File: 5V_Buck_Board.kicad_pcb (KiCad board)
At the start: 2 copper layers, 97.1 x 70 mm, 10 parts, among them J1 XT60PW-M, J2 XT60PW-F

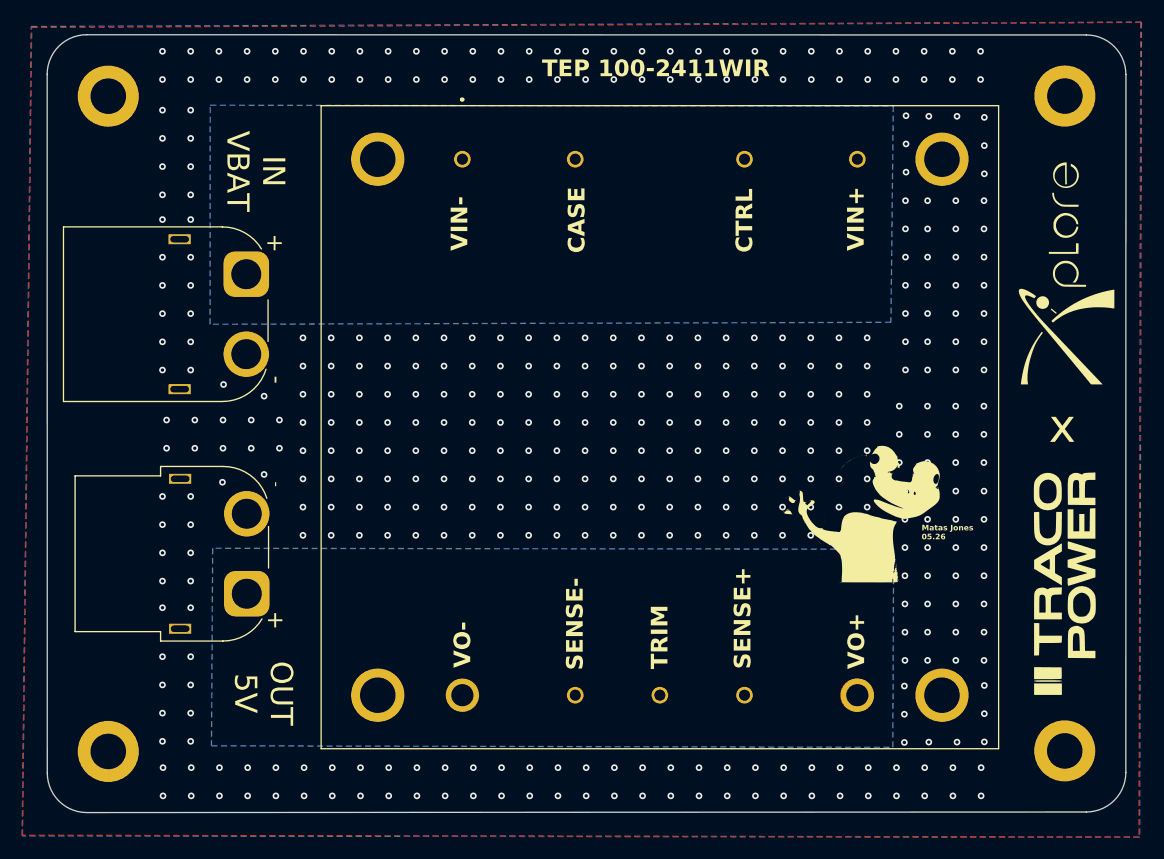
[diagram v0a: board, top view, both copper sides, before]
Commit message: Board ready for REV2
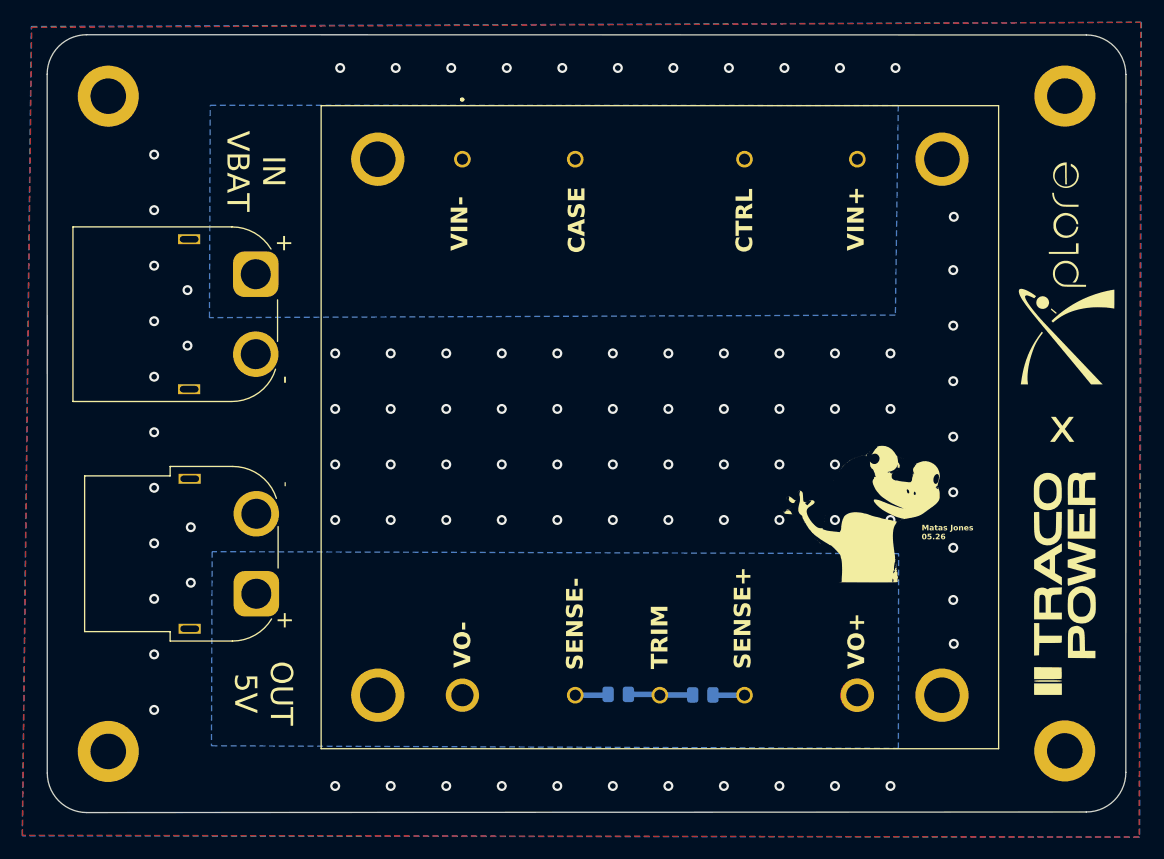
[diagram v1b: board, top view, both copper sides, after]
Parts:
- added R1: NM, Resistor_SMD:R_0805_2012Metric, B.Cu at (159.4, 118.2)
- added R2: NM, Resistor_SMD:R_0805_2012Metric, B.Cu at (151.8, 118.2)
- moved J2 0.86 mm to (119.2, 101.9)
- moved J1 0.86 mm to (119.2, 87.5)
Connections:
- PS1 pad 7: unconnected-(PS1-TRIM-Pad7) -> Net-(PS1-TRIM)
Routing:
- net Net-(PS1-TRIM): track 0.00 -> 5.83 mm
- net GND: track 0.00 -> 2.99 mm, vias 424 -> 90
- net Net-(PS1-+SENSE): track 0.05 -> 2.90 mm
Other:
- board text removed: "TEP 100-2411WIR"

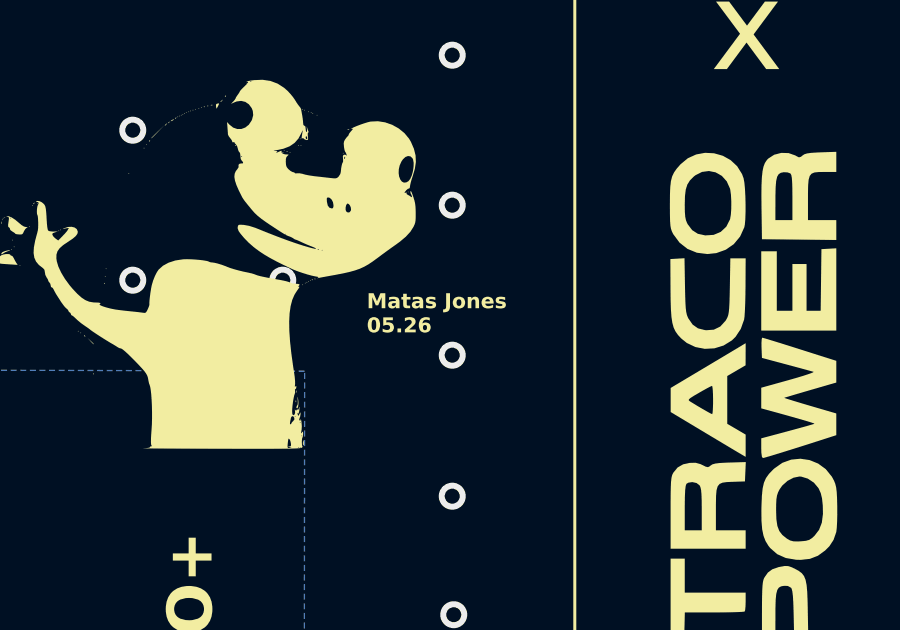
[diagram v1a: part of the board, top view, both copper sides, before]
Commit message: Added Pedro's name
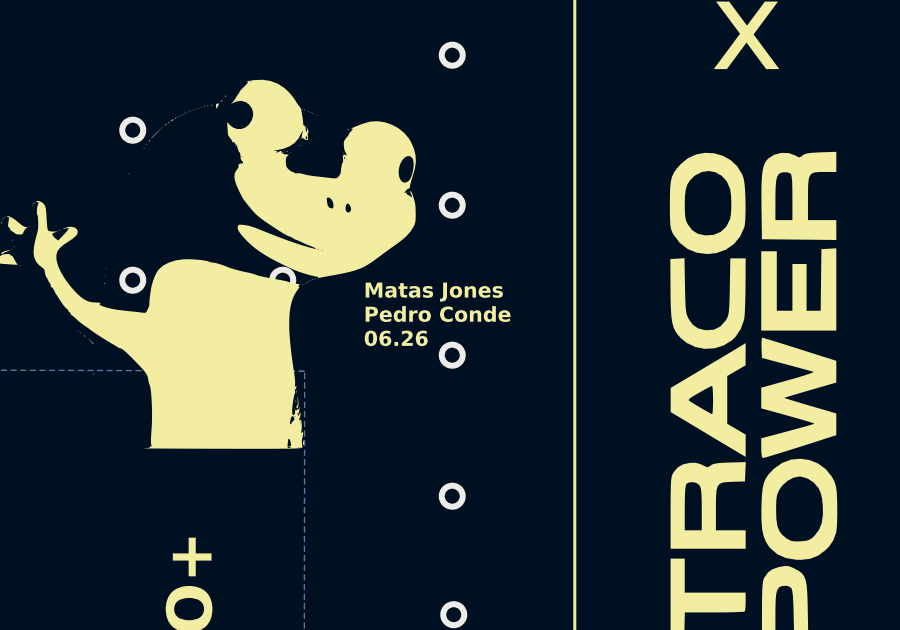
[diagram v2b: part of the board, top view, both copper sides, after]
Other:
- board text added: "Matas Jones Pedro Conde 06.26"
- board text removed: "Matas Jones 05.26"
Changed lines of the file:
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@@
 		)
 	)
-	(gr_text "Matas Jones\n05.26"
-		(at 179.1 104.25 0)
+	(gr_text "Matas Jones\nPedro Conde\n06.26"
+		(at 179 104.7 0)
 		(layer "F.SilkS")
 		(effects
